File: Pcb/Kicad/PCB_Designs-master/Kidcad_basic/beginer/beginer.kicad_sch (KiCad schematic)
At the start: 16 parts, among them J1 PINHD_1x1_Female, J10 PINHD_1x1_Female, J11 PINHD_1x1_Female, J12 PINHD_1x1_Female, J2 PINHD_1x1_Female, J3 PINHD_1x1_Female, J4 PINHD_1x1_Female, J5 PINHD_1x1_Female, J6 PINHD_1x1_Female, J7 PINHD_1x1_Female, J8 PINHD_1x1_Female, J9 PINHD_1x1_Female, SW1 SW_DPDT_x2

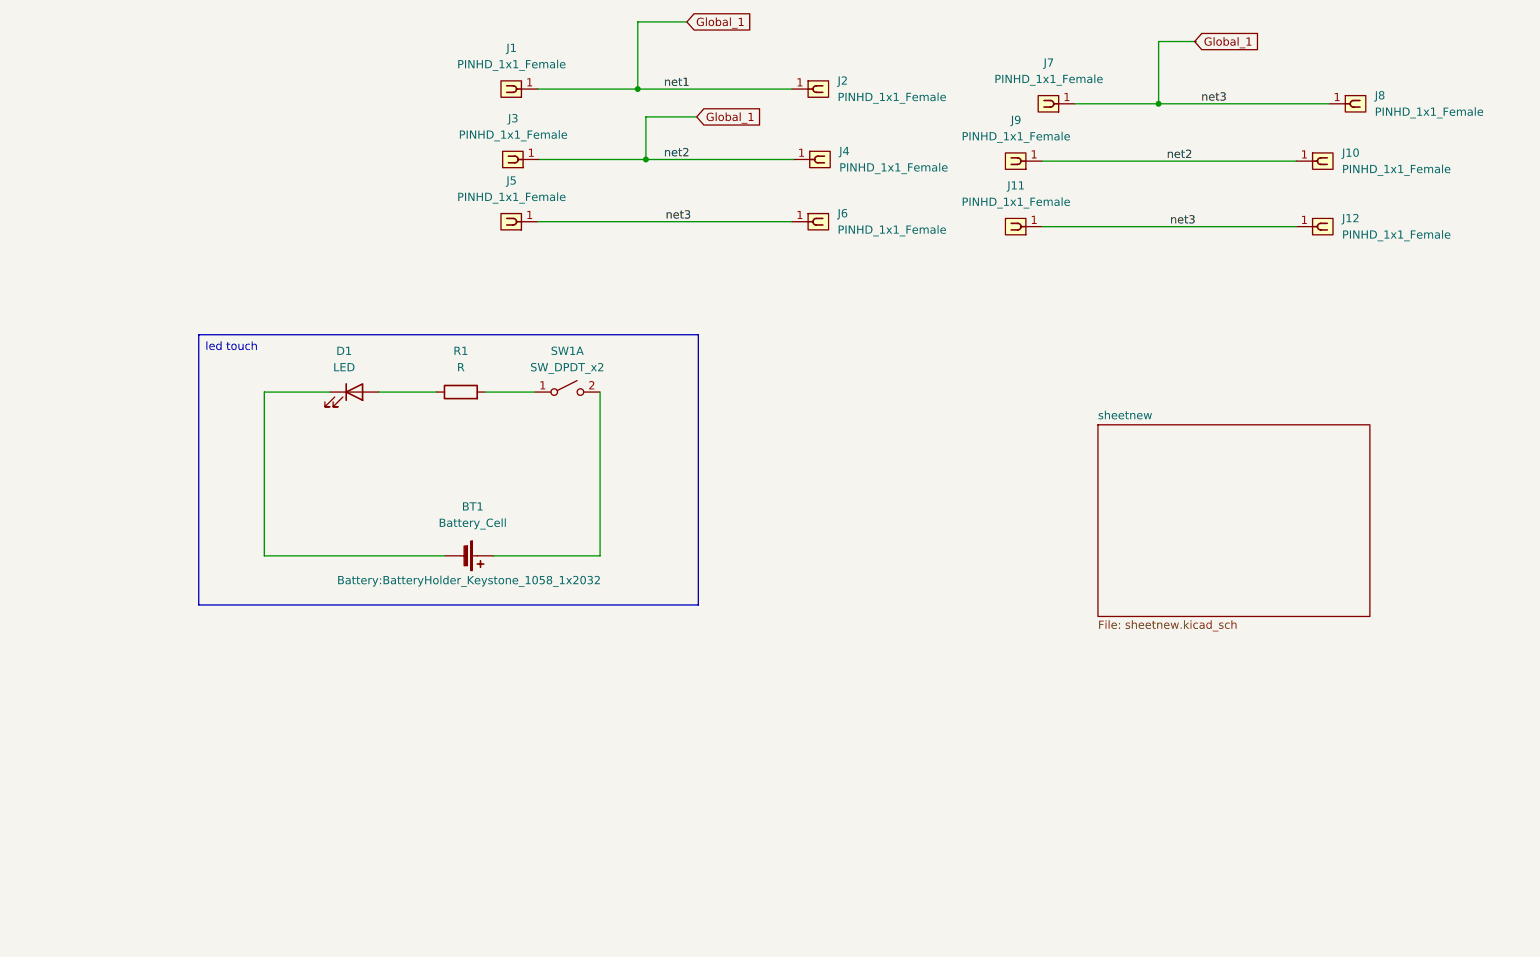
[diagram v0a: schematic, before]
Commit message: update file kicad
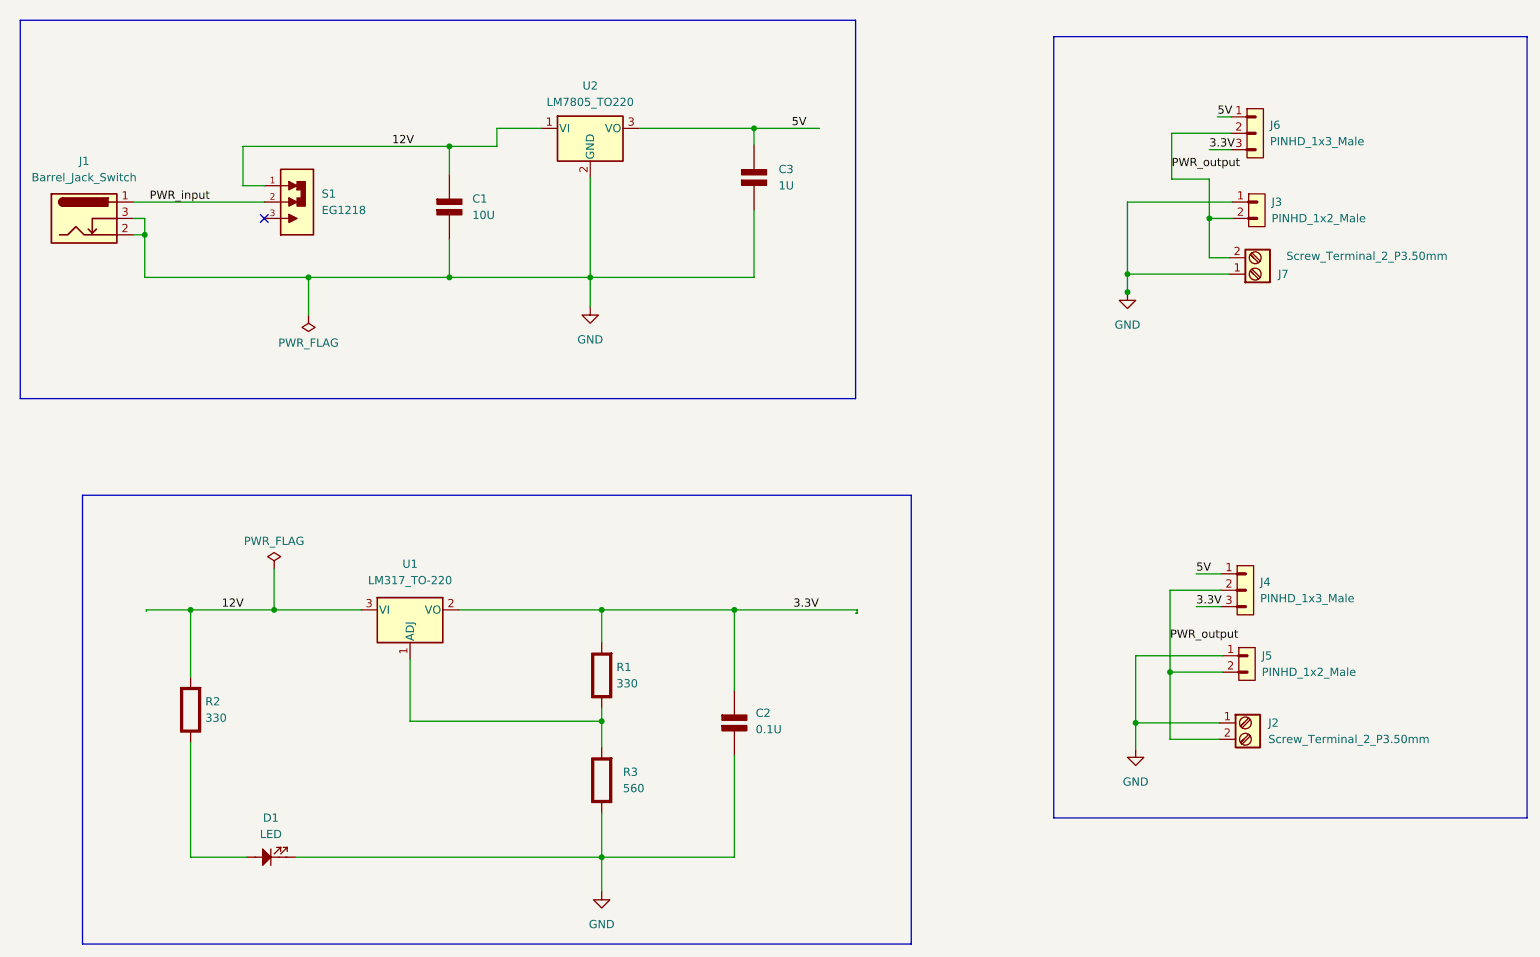
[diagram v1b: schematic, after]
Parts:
- removed BT1: Battery_Cell, Battery:BatteryHolder_Keystone_1058_1x2032, symbol Device:Battery_Cell
- removed D1: LED, LED_THT:LED_D5.0mm, symbol Device:LED
- removed J1, J10, J11, J12, J2, J3, J4, J5, J6, J7, J8, J9: PINHD_1x1_Female, Connector_PinSocket_2.54mm:PinSocket_1x01_P2.54mm_Vertical, symbol PCM_SL_Pin_Headers:PINHD_1x1_Female
- removed R1: R, Resistor_THT:R_Axial_DIN0204_L3.6mm_D1.6mm_P7.62mm_Horizontal, symbol Device:R
- removed SW1: SW_DPDT_x2, Button_Switch_THT:SW_TH_Tactile_Omron_B3F-10xx, symbol Switch:SW_DPST_x2
- added C1: 10U, Capacitor_THT:C_Disc_D3.0mm_W1.6mm_P2.50mm, symbol PCM_Elektuur:C
- added C2: 0.1U, Capacitor_THT:C_Disc_D3.0mm_W1.6mm_P2.50mm, symbol PCM_Elektuur:C
- added C3: 1U, Capacitor_THT:C_Disc_D3.0mm_W1.6mm_P2.50mm, symbol PCM_Elektuur:C
- added D1: LED, LED_THT:LED_D5.0mm, symbol PCM_SL_Devices:LED
- added J1: Barrel_Jack_Switch, Connector_BarrelJack:BarrelJack_Horizontal, symbol Connector:Barrel_Jack_Switch
- added J2, J7: Screw_Terminal_2_P3.50mm, TerminalBlock_Phoenix:TerminalBlock_Phoenix_PT-1,5-2-3.5-H_1x02_P3.50mm_Horizontal, symbol PCM_SL_Screw_Terminal:Screw_Terminal_2_P3.50mm
- added J3, J5: PINHD_1x2_Male, Connector_PinHeader_2.54mm:PinHeader_1x02_P2.54mm_Vertical, symbol PCM_SL_Pin_Headers:PINHD_1x2_Male
- added J4, J6: PINHD_1x3_Male, Connector_PinHeader_2.54mm:PinHeader_1x03_P2.54mm_Vertical, symbol PCM_SL_Pin_Headers:PINHD_1x3_Male
- added R1, R2: 330, Resistor_THT:R_Axial_DIN0204_L3.6mm_D1.6mm_P7.62mm_Horizontal, symbol PCM_Elektuur:R
- added R3: 560, Resistor_THT:R_Axial_DIN0204_L3.6mm_D1.6mm_P7.62mm_Horizontal, symbol PCM_Elektuur:R
- added S1: EG1218, EG1218:SW_EG1218, symbol EG1218:EG1218
- added U1: LM317_TO-220, Package_TO_SOT_THT:TO-220-3_Vertical, symbol Regulator_Linear:LM317_TO-220
- added U2: LM7805_TO220, Package_TO_SOT_THT:TO-220-3_Vertical, symbol Regulator_Linear:LM7805_TO220
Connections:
- new net: R1.1 (+), R3.2 (-), U1.1 (ADJ)
- new net: D1.2, R2.1 (+)
- new net 12V: C1.1 (+), R2.2 (-), S1.1, U1.3 (VI), U2.1 (VI)
- new net 3.3V: C2.1 (+), J4.3, J6.3, R1.2 (-), U1.2 (VO)
- new net 5V: C3.1 (+), J4.1, J6.1, U2.3 (VO)
- new net GND: C1.2 (-), C2.2 (-), C3.2 (-), D1.1, J1.2, J1.3, J2.1, J3.1, J5.1, J7.1, R3.1 (+), U2.2 (GND)
- new net PWR_input: J1.1, S1.2
- new net PWR_output: J2.2, J3.2, J4.2, J5.2, J6.2, J7.2
- no-connect marks 0 -> 1
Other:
- removed sheet sheetnew
